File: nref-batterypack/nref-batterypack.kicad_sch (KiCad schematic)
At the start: 48 parts, among them J1 C3+, J2 DBG, J3 PACK_CONN, J4 C4+, J5 C2+, J6 C1+, J7 C1-, SW1 Reset, U1 BQ76905, U2 TPS259482, U3 MSPM0L130xRGE

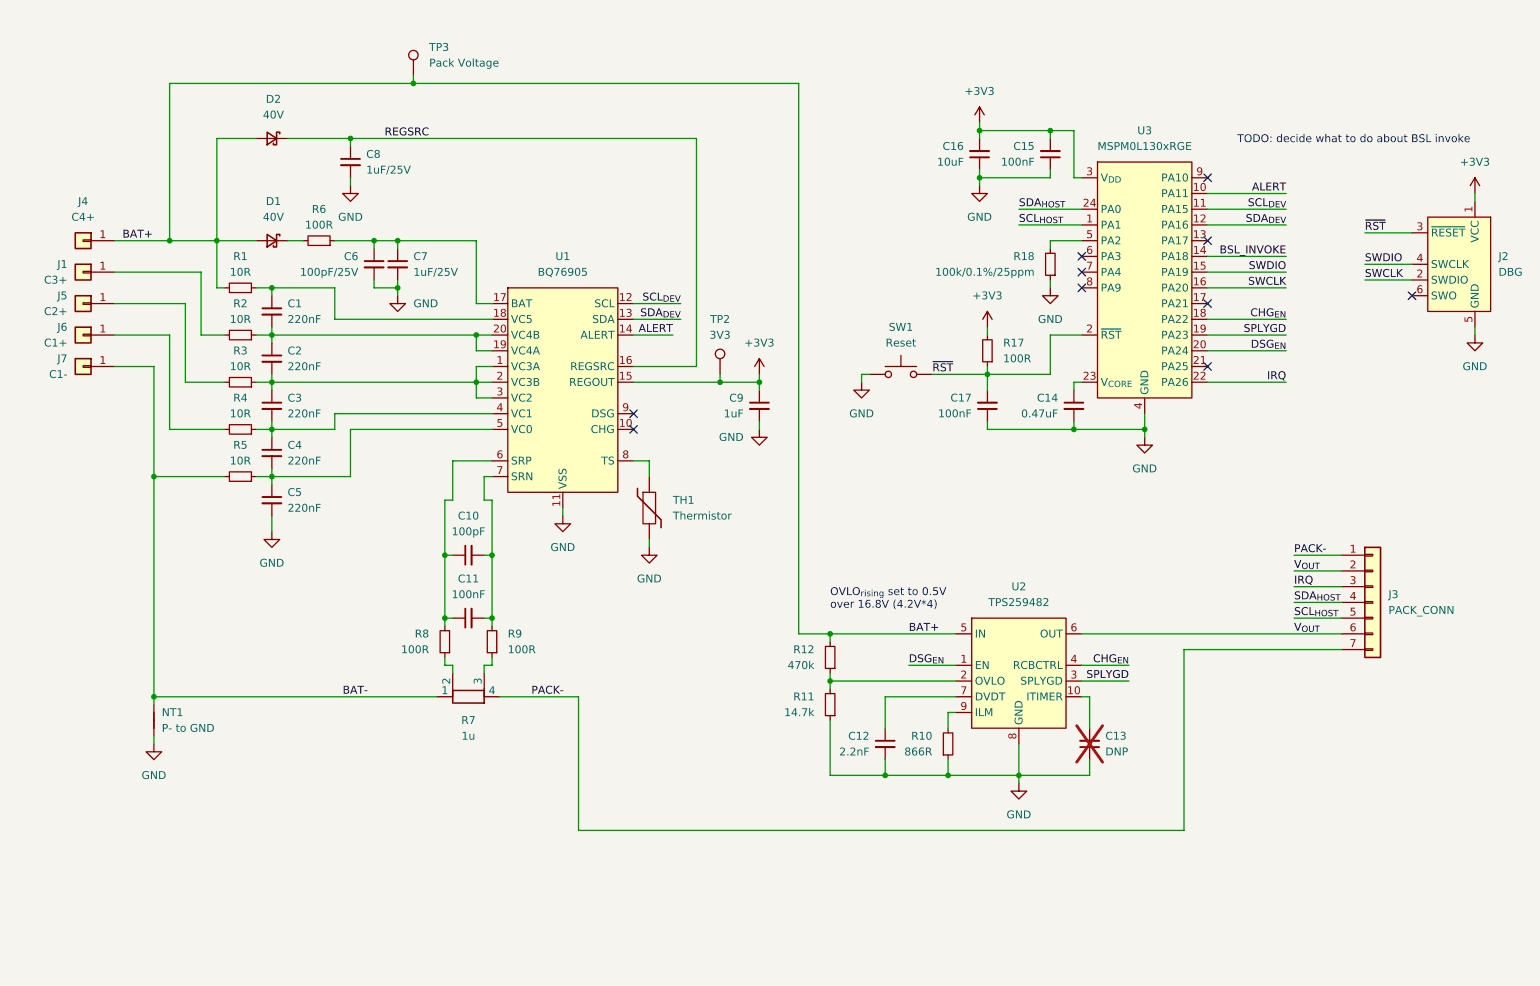
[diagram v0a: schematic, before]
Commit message: wip of the new version with another bms ic
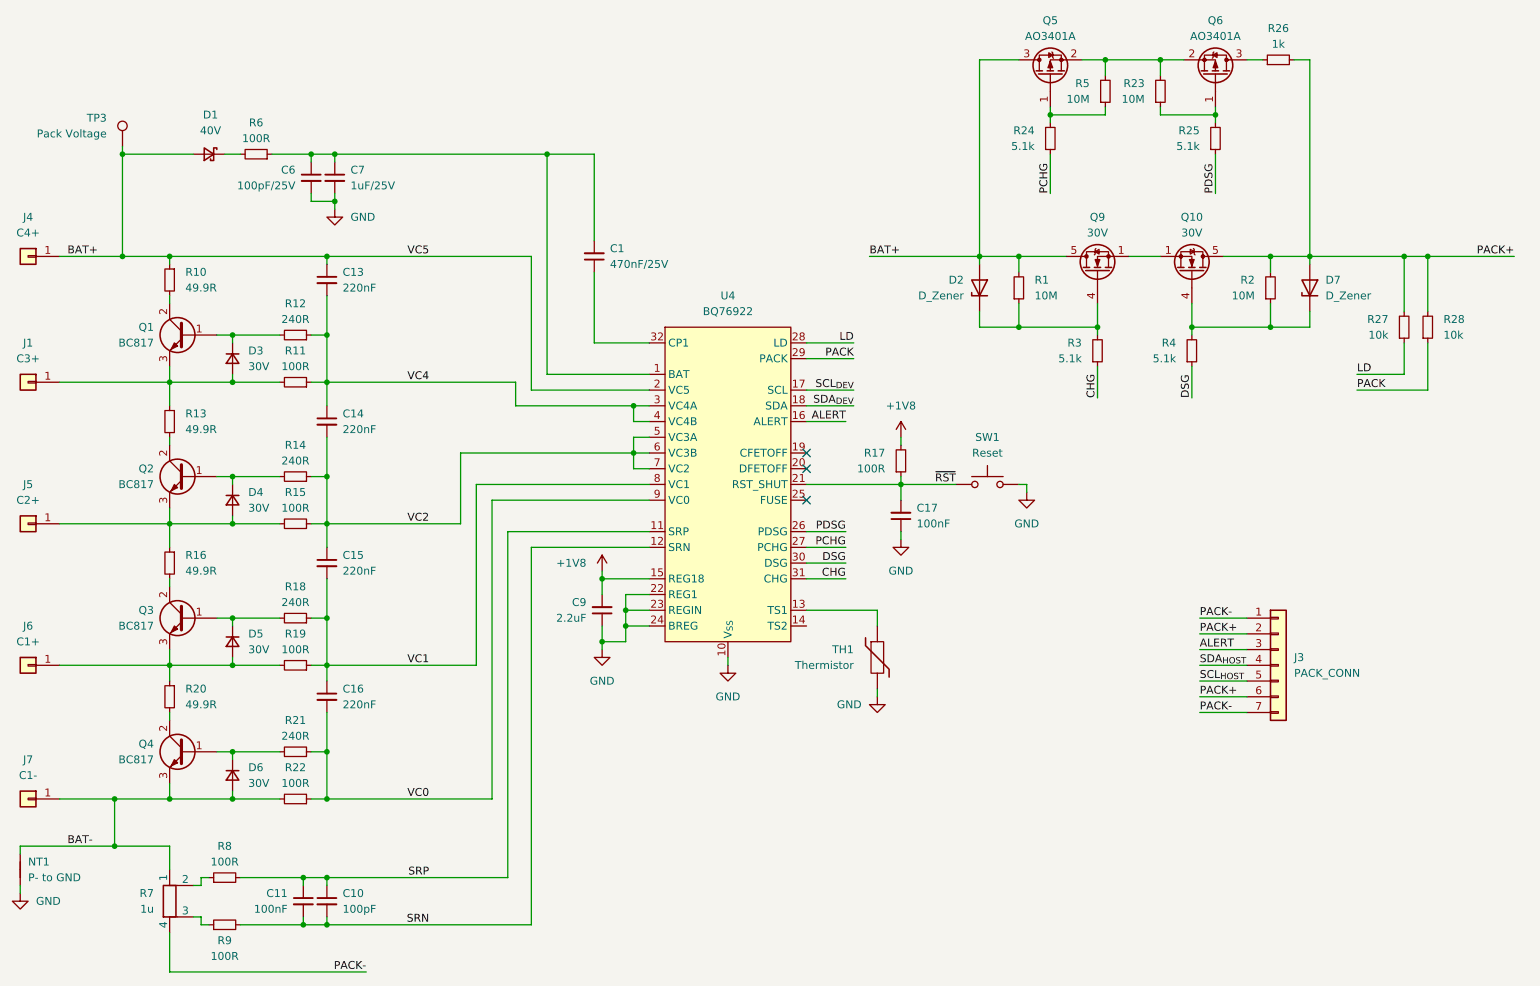
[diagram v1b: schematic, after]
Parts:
- removed C12: 2.2nF, Capacitor_SMD:C_0402_1005Metric, symbol Device:C_Small
- removed C2, C3, C4, C5: 220nF, Capacitor_SMD:C_0603_1608Metric, symbol Device:C_Small
- removed C8: 1uF/25V, Capacitor_SMD:C_0603_1608Metric, symbol Device:C_Small
- removed D2: 40V, Diode_SMD:D_SOD-323, symbol Device:D_Schottky_Small
- removed J2: DBG, Connector:Tag-Connect_TC2030-IDC-NL_2x03_P1.27mm_Vertical, symbol Connector:Conn_ARM_SWD_TagConnect_TC2030-NL
- removed TP2: 3V3, TestPoint:TestPoint_Pad_1.5x1.5mm, symbol Connector:TestPoint
- removed U1: BQ76905, Package_DFN_QFN:QFN-20-1EP_3.5x3.5mm_P0.5mm_EP2x2mm_ThermalVias, symbol meansOfCircuitDesign:BQ76905
- removed U2: TPS259482, Automated:PowerWCSP12_YWP_TEX, symbol meansOfCircuitDesign:TPS25948x
- removed U3: MSPM0L130xRGE, Package_DFN_QFN:VQFN-24-1EP_4x4mm_P0.5mm_EP2.5x2.5mm_ThermalVias, symbol meansOfCircuitDesign:MSPM0L130xRGE
- added D2, D7: D_Zener, symbol Device:D_Zener
- added D3, D4, D5, D6: 30V, Diode_SMD:D_SOD-323F, symbol Device:D_Small
- added Q1, Q2, Q3, Q4: BC817, Package_TO_SOT_SMD:SOT-23, symbol Device:Q_NPN_BCE
- added Q10, Q9: 30V, Package_SON:Diodes_PowerDI3333-8, symbol Transistor_FET:DMN3008SFG
- added Q5, Q6: AO3401A, Package_TO_SOT_SMD:SOT-23, symbol Transistor_FET:AO3401A
- added R13, R16, R20: 49.9R, Resistor_SMD:R_1206_3216Metric, symbol Device:R_Small
- added R14, R21: 240R, Resistor_SMD:R_0603_1608Metric, symbol Device:R_Small
- added R15, R19, R22: 100R, Resistor_SMD:R_0603_1608Metric, symbol Device:R_Small
- added R23: 10M, Resistor_SMD:R_0603_1608Metric, symbol Device:R_Small
- added R24, R25: 5.1k, Resistor_SMD:R_0603_1608Metric, symbol Device:R_Small
- added R26: 1k, Resistor_SMD:R_1206_3216Metric, symbol Device:R_Small
- added R27, R28: 10k, Resistor_SMD:R_0603_1608Metric, symbol Device:R_Small
- added U4: BQ76922, Package_DFN_QFN:Texas_RSN_WQFN-32-1EP_4x4mm_P0.4mm_EP2.8x2.8mm, symbol meansOfCircuitDesign:BQ76922
- C1: value 220nF -> 470nF/25V
- C13: value DNP -> 220nF; footprint Capacitor_SMD:C_0402_1005Metric -> Capacitor_SMD:C_0603_1608Metric; now fitted
- C14: value 0.47uF -> 220nF; footprint Capacitor_SMD:C_0402_1005Metric -> Capacitor_SMD:C_0603_1608Metric
- C15: value 100nF -> 220nF; footprint Capacitor_SMD:C_0402_1005Metric -> Capacitor_SMD:C_0603_1608Metric
- C16: value 10uF -> 220nF
- C9: value 1uF -> 2.2uF
- R1, R2, R5: value 10R -> 10M; footprint Resistor_SMD:R_1206_3216Metric -> Resistor_SMD:R_0603_1608Metric
- R10: value 866R -> 49.9R; footprint Resistor_SMD:R_0402_1005Metric -> Resistor_SMD:R_1206_3216Metric
- R11: value 14.7k -> 100R; footprint Resistor_SMD:R_0402_1005Metric -> Resistor_SMD:R_0603_1608Metric
- R12: value 470k -> 240R; footprint Resistor_SMD:R_0402_1005Metric -> Resistor_SMD:R_0603_1608Metric
- R18: value 100k/0.1%/25ppm -> 240R; footprint Resistor_SMD:R_0402_1005Metric -> Resistor_SMD:R_0603_1608Metric
- R3, R4: value 10R -> 5.1k; footprint Resistor_SMD:R_1206_3216Metric -> Resistor_SMD:R_0603_1608Metric
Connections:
- net IRQ is gone; now on net ALERT: J3.3 (Pin_3)
- net V_{OUT} is gone; now on net PACK+: J3.2 (Pin_2), J3.6 (Pin_6)
- net ALERT: now also U4.16 (ALERT)
- net BAT-: now also D6.2 (A), Q4.3 (E), R22.2; no longer R5.2
- net GND: now also C9.1, U4.10 (V_{SS}), U4.22 (REG1), U4.23 (REGIN), U4.24 (BREG), U4.33 (EP); no longer C13.1, C14.2, C15.1, C16.1, C9.2, R10.1, R11.1, R18.1
- net SCL_{DEV}: now also U4.17 (SCL)
- net SDA_{DEV}: now also U4.18 (SDA)
- net ~{RST}: now also U4.21 (RST_SHUT)
- net at C1.2: now also C6.1, C7.1, R6.1, U4.1 (BAT); no longer R2.1
- net CHG: now reaches R3.1
- net CHG: now also U4.31 (CHG)
- net SRP: now reaches C10.1, C11.1, R8.2
- net SRP: now also U4.11 (SRP)
- net at R5.1: now also Q5.1 (G), R24.2
- net at R11.2: now also J1.1 (Pin_1), D3.2 (A), Q1.3 (E), R13.1; no longer R12.1
- net VC4: now reaches C14.1
- net VC4: now also C13.2, R11.1, R12.1, U4.3 (VC4A), U4.4 (VC4B)
- net at R3.2: now also R1.1, D2.1 (K), Q9.4 (G); no longer J5.1 (Pin_1)
- net SRN: now reaches C10.2, C11.2, R9.2
- net SRN: now also U4.12 (SRN)
- net DSG: now reaches R4.1
- net DSG: now also U4.30 (DSG)
- net at J6.1 (Pin_1): now also D5.2 (A), Q3.3 (E), R19.2, R20.1; no longer R4.2
- net PACK+: now reaches R2.2
- net PACK+: now also D7.2 (A), Q10.5 (D), R26.2, R27.2, R28.2; no longer J1.1 (Pin_1)
- net at C1.1: now also U4.32 (CP1); no longer R1.1
- net at TH1.1: now also U4.13 (TS1)
- net at R10.2: now also Q1.2 (C)
- net at R18.2: now also D5.1 (K), Q3.1 (B)
- removed net +3V3: C15.2, C16.2, C9.1, R17.2
- net IN renamed BAT+
- net BAT+: now also C13.1, R10.1, D2.2 (A), Q5.3 (D), Q9.5 (D), U4.2 (VC5); no longer R12.2
- new net: Q10.1 (S), Q10.2 (S), Q10.3 (S), Q9.1 (S), Q9.2 (S), Q9.3 (S)
- new net: D6.1 (K), Q4.1 (B), R21.2
- new net: Q4.2 (C), R20.2
- new net: Q5.2 (S), Q6.2 (S), R23.2, R5.2
- new net: Q2.2 (C), R13.2
- new net: D4.2 (A), J5.1 (Pin_1), Q2.3 (E), R15.2, R16.1
- new net: Q3.2 (C), R16.2
- new net: D3.1 (K), Q1.1 (B), R12.2
- new net: D7.1 (K), Q10.4 (G), R2.1, R4.2
- new net: Q6.1 (G), R23.1, R25.2
- new net: Q6.3 (D), R26.1
- new net: D4.1 (K), Q2.1 (B), R14.2
- new net +1V8: C9.2, R17.2, U4.15 (REG18)
- new net LD: R27.1, U4.28 (LD)
- new net PACK: R28.1, U4.29 (PACK)
- new net PCHG: R24.1, U4.27 (PCHG)
- new net PDSG: R25.1, U4.26 (PDSG)
- new net VC0: C16.2, R21.1, R22.1, U4.9 (VC0)
- new net VC1: C15.2, C16.1, R18.1, R19.1, U4.8 (VC1)
- new net VC2: C14.2, C15.1, R14.1, R15.1, U4.5 (VC3A), U4.6 (VC3B), U4.7 (VC2)
- no-connect marks 10 -> 3
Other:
- note removed: "OVLO_{rising} set to 0.5V over 16.8V (4.2V*4)"
- note removed: "TODO: decide what to do about BSL invoke"
- moved on the sheet: C10, C11, C17, C6, C7, D1, J1, J3, J4, J5, J6, J7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
